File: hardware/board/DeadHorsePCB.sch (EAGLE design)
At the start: 23 parts, among them J1 DIN5, Q1 BSS138, Q2 BSS138

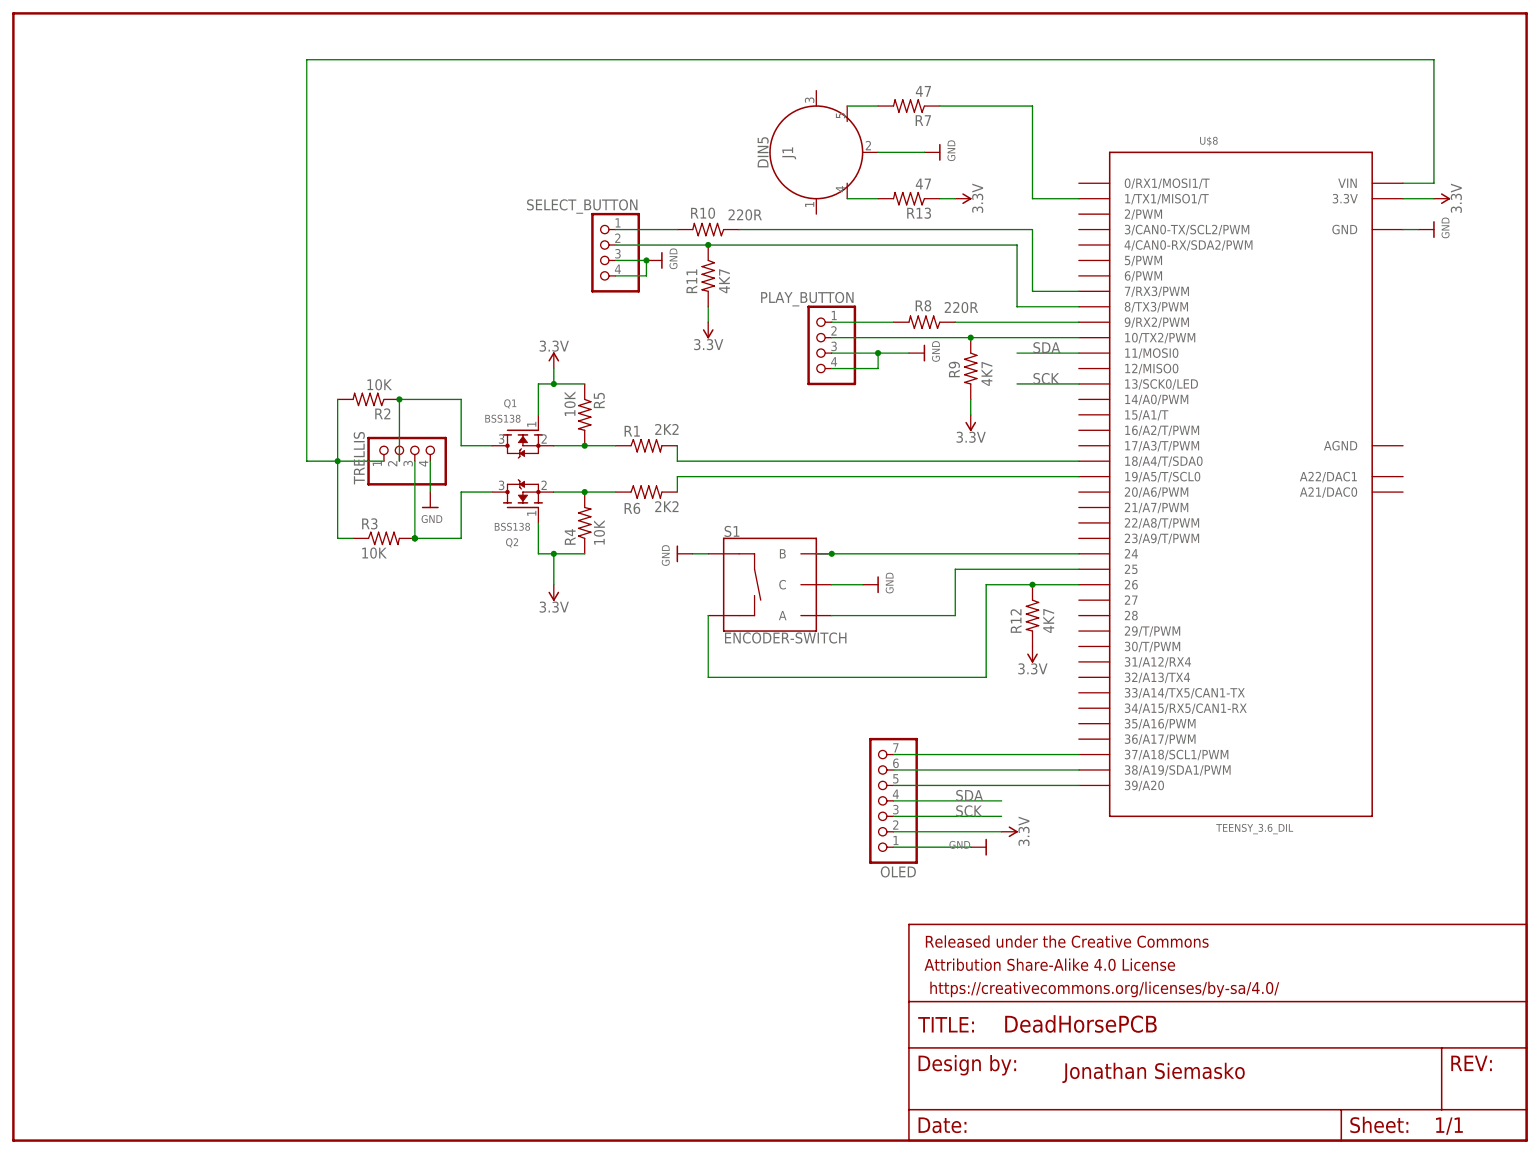
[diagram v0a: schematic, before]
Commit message: Getting closer on the PCB
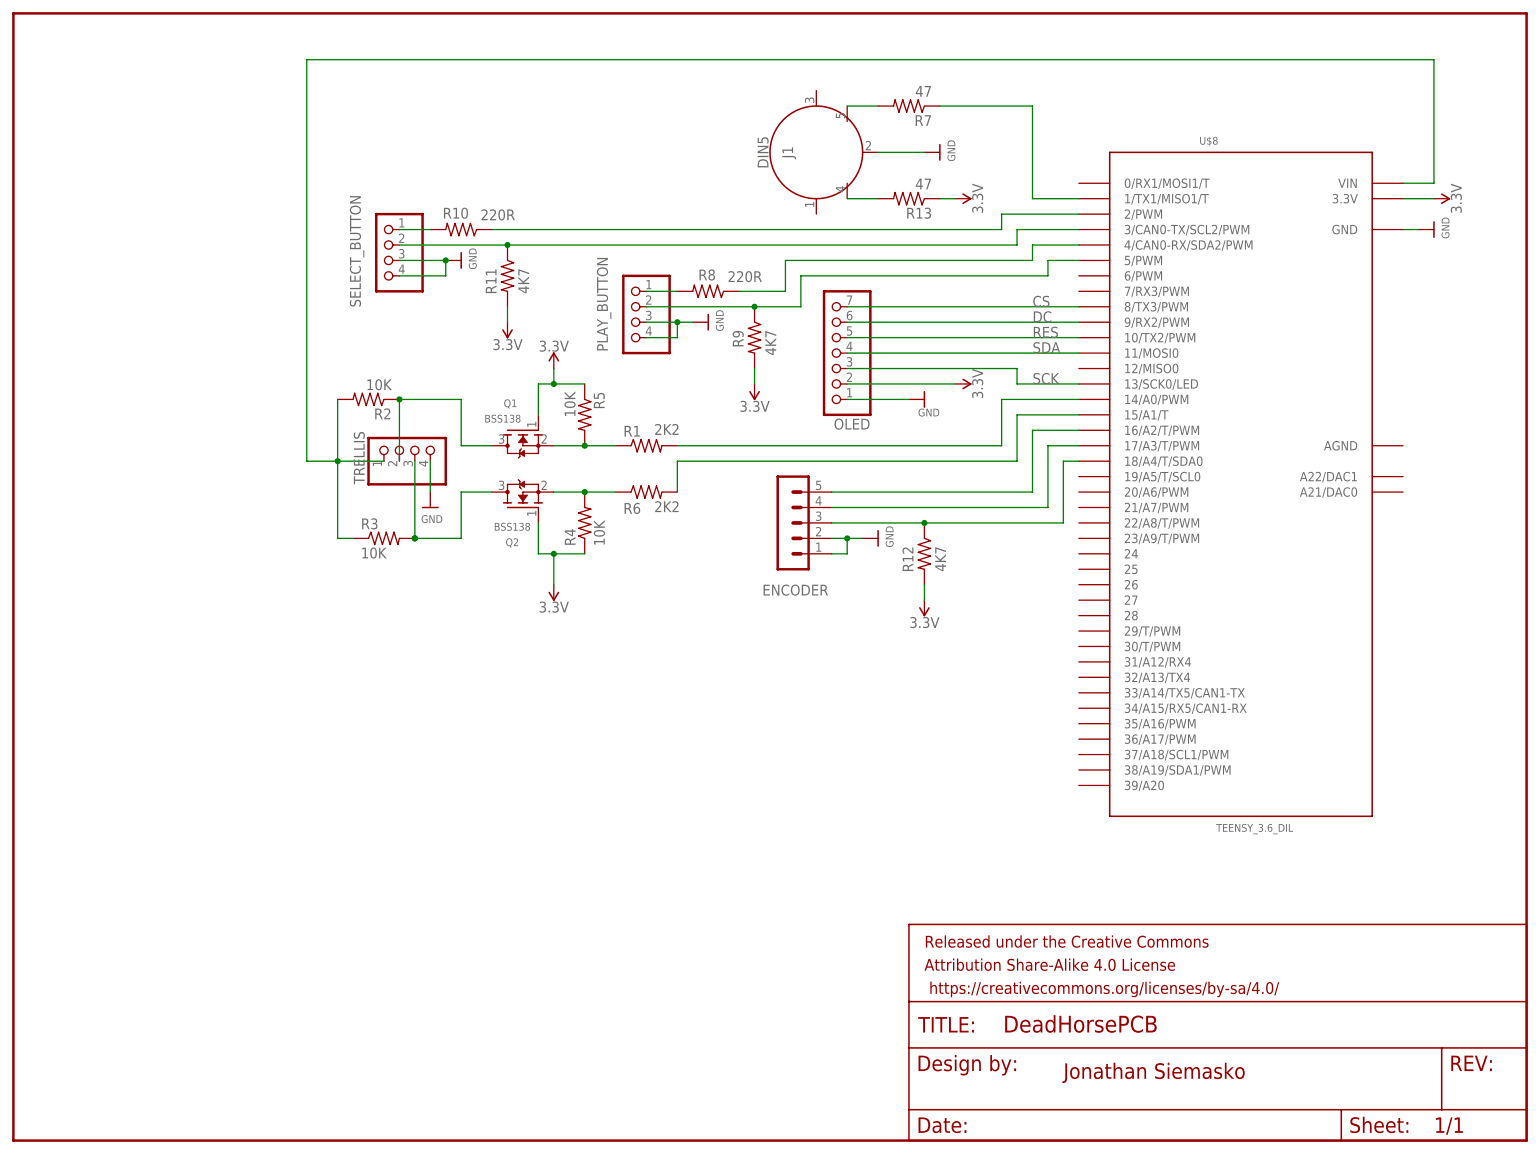
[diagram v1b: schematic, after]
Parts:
- removed S1: ENCODER-SWITCH, SparkFun-Switches:ENCODER-SWITCH
- added ENCODER: (no value), con-lstb:MA05-1
- PLAY_BUTTON: value PlayButton -> PlayBtn
- SELECT_BUTTON: value SelectButton -> SelectBtn
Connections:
- removed net N$11: OLED.5, U$8.39/A20
- removed net N$15: S1.B, U$8.24
- removed net N$17: S1.A, U$8.25
- removed net N$19: R11.1, SELECT_BUTTON.2, U$8.8/TX3/PWM
- new net CS: OLED.7, U$8.8/TX3/PWM
- new net DC: OLED.6, U$8.9/RX2/PWM
- new net N$22: R11.1, SELECT_BUTTON.2, U$8.3/CAN0-TX/SCL2/PWM
- new net RES: OLED.5, U$8.10/TX2/PWM
- net GND: now also ENCODER.1, ENCODER.2; no longer S1.C, S1.SW+
- net N$10: now also ENCODER.5, U$8.16/A2/T/PWM; no longer OLED.6, U$8.38/A19/SDA1/PWM
- net N$13: now also U$8.4/CAN0-RX/SDA2/PWM; no longer U$8.9/RX2/PWM
- net N$14: now also U$8.5/PWM; no longer U$8.10/TX2/PWM
- net N$16: now also U$8.2/PWM; no longer U$8.7/RX3/PWM
- net N$20: now also ENCODER.3, U$8.18/A4/T/SDA0; no longer S1.SW-, U$8.26
- net N$6: now also U$8.14/A0/PWM; no longer U$8.18/A4/T/SDA0
- net N$7: now also U$8.15/A1/T; no longer U$8.19/A5/T/SCL0
- net N$9: now also ENCODER.4, U$8.17/A3/T/PWM; no longer OLED.7, U$8.37/A18/SCL1/PWM
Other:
- moved on the sheet: OLED, PLAY_BUTTON, R10, R11, R12, R8, R9, SELECT_BUTTON

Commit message: Added Ground Plane
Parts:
- ENCODER: value (none) -> ENCODER
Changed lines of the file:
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@@
 <part name="U$4" library="microbuilder" deviceset="GND" device=""/>
 <part name="SUPPLY8" library="SparkFun-PowerSymbols" deviceset="3.3V" device=""/>
-<part name="ENCODER" library="con-lstb" library_urn="urn:adsk.eagle:library:162" deviceset="MA05-1" device="" package3d_urn="urn:adsk.eagle:package:8332/1"/>
+<part name="ENCODER" library="con-lstb" library_urn="urn:adsk.eagle:library:162" deviceset="MA05-1" device="" package3d_urn="urn:adsk.eagle:package:8332/1" value="ENCODER"/>
 </parts>
 <sheets>
@@
 <instance part="SUPPLY8" gate="G$1" x="154.94" y="-30.48" rot="R270"/>
 <instance part="ENCODER" gate="G$1" x="127" y="-83.82" smashed="yes">
-<attribute name="VALUE" x="125.73" y="-93.98" size="1.778" layer="96"/>
 <attribute name="NAME" x="123.19" y="-95.758" size="1.778" layer="95"/>
 </instance>
